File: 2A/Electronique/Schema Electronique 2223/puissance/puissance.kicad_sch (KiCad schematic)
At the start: 19 parts, among them J101 Bat 2, J102 Bat 1, J103 AU, J104 Switch, J15 Conn_02x20_Odd_Even

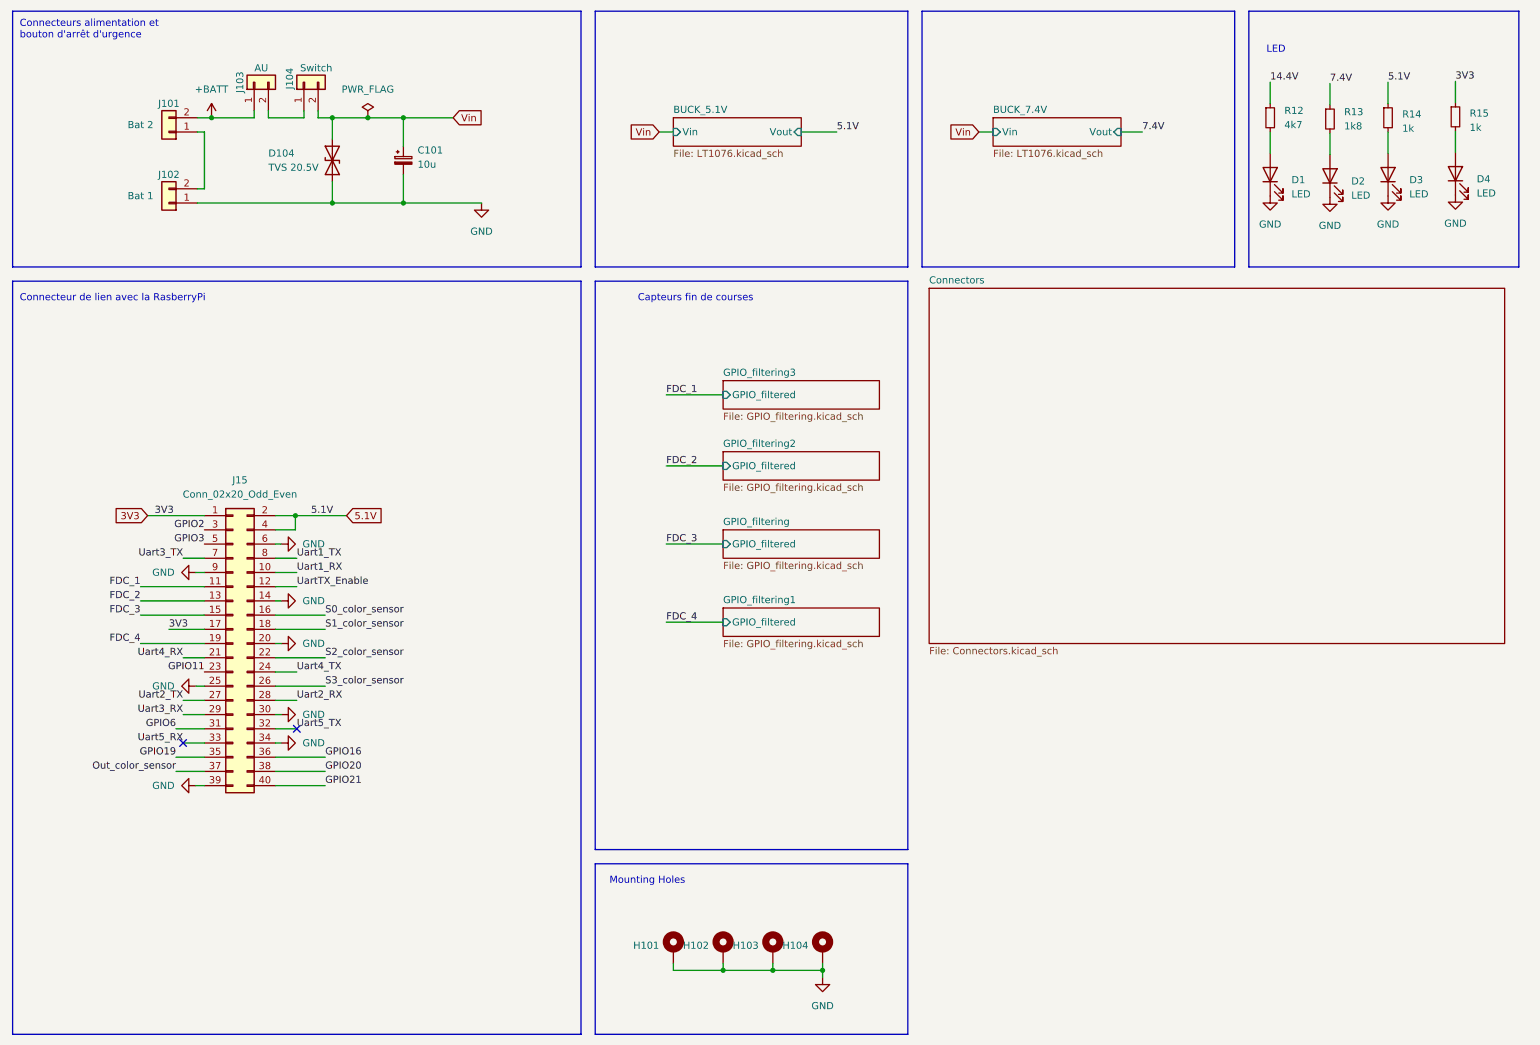
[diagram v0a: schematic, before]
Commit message: update puissance
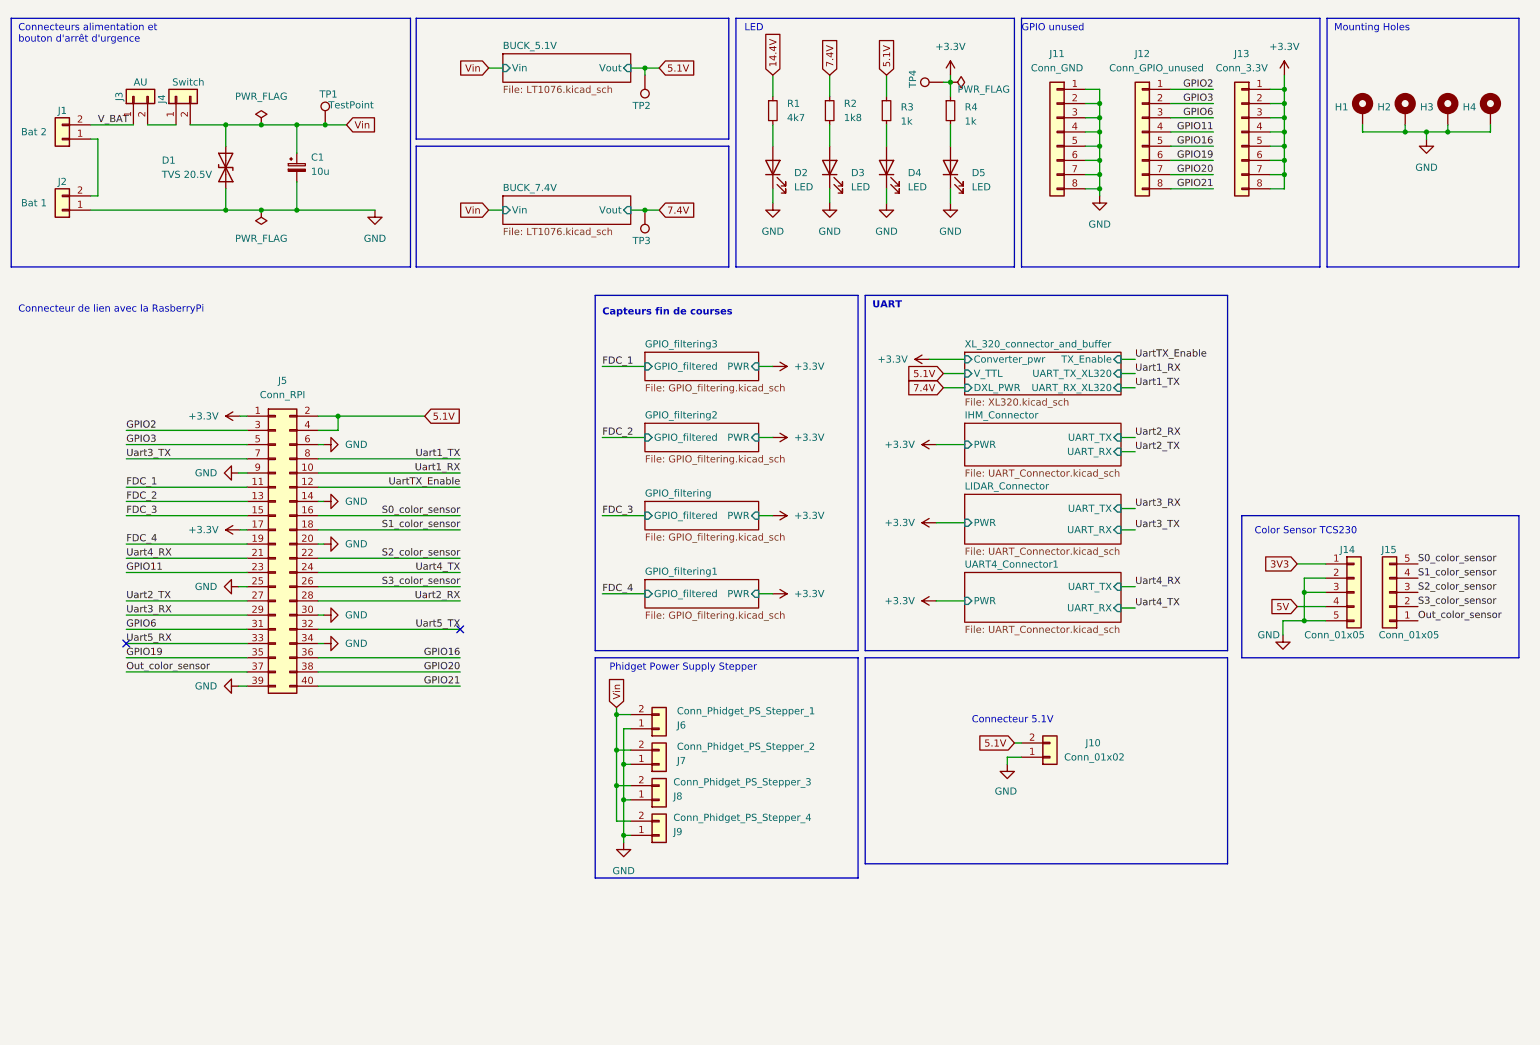
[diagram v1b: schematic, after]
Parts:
- removed C101: 10u, Capacitor_SMD:CP_Elec_5x5.4, symbol Device:C_Polarized_Small
- removed D1: LED, LED_SMD:LED_0603_1608Metric_Pad1.05x0.95mm_HandSolder, symbol Device:LED
- removed D104: TVS 20.5V, symbol Diode:1.5KExxCA
- removed H101, H102, H103, H104: MountingHole_Pad, MountingHole:MountingHole_3.2mm_M3_Pad_Via, symbol Mechanical:MountingHole_Pad
- removed J101: Bat 2, symbol Connector_Generic:Conn_01x02
- removed J102: Bat 1, symbol Connector_Generic:Conn_01x02
- removed J103: AU, symbol Connector_Generic:Conn_01x02
- removed J104: Switch, symbol Connector_Generic:Conn_01x02
- removed J15: Conn_02x20_Odd_Even, symbol Connector_Generic:Conn_02x20_Odd_Even
- removed R12: 4k7, Resistor_SMD:R_0603_1608Metric_Pad0.98x0.95mm_HandSolder, symbol Device:R_Small
- removed R13: 1k8, Resistor_SMD:R_0603_1608Metric_Pad0.98x0.95mm_HandSolder, symbol Device:R_Small
- removed R14, R15: 1k, Resistor_SMD:R_0603_1608Metric_Pad0.98x0.95mm_HandSolder, symbol Device:R_Small
- added C1: 10u, Capacitor_SMD:CP_Elec_4x5.4, symbol Device:C_Polarized_Small
- added D1: TVS 20.5V, Diode_SMD:D_SMB, symbol Diode:1.5KExxCA
- added D5: LED, LED_SMD:LED_0603_1608Metric, symbol Device:LED
- added H1, H2, H3, H4: MountingHole_Pad, MountingHole:MountingHole_2.7mm_M2.5_Pad_Via, symbol Mechanical:MountingHole_Pad
- added J1: Bat 2, custom:691322110002, symbol Connector_Generic:Conn_01x02
- added J10: Conn_01x02, Connector_JST:JST_XH_B2B-XH-A_1x02_P2.50mm_Vertical, symbol Connector_Generic:Conn_01x02
- added J11: Conn_GND, Connector_PinHeader_2.54mm:PinHeader_1x08_P2.54mm_Vertical, symbol Connector_Generic:Conn_01x08
- added J12: Conn_GPIO_unused, Connector_PinHeader_2.54mm:PinHeader_1x08_P2.54mm_Vertical, symbol Connector_Generic:Conn_01x08
- added J13: Conn_3.3V, Connector_PinHeader_2.54mm:PinHeader_1x08_P2.54mm_Vertical, symbol Connector_Generic:Conn_01x08
- added J14, J15: Conn_01x05, Connector_JST:JST_XH_B5B-XH-A_1x05_P2.50mm_Vertical, symbol Connector_Generic:Conn_01x05
- added J2: Bat 1, custom:691322110002, symbol Connector_Generic:Conn_01x02
- added J3: AU, custom:691322110002, symbol Connector_Generic:Conn_01x02
- added J4: Switch, custom:691322110002, symbol Connector_Generic:Conn_01x02
- added J5: Conn_RPI, Connector_PinSocket_2.54mm:PinSocket_2x20_P2.54mm_Vertical, symbol Connector_Generic:Conn_02x20_Odd_Even
- added J6: Conn_Phidget_PS_Stepper_1, Connector_JST:JST_XH_B2B-XH-A_1x02_P2.50mm_Vertical, symbol Connector_Generic:Conn_01x02
- added J7: Conn_Phidget_PS_Stepper_2, Connector_JST:JST_XH_B2B-XH-A_1x02_P2.50mm_Vertical, symbol Connector_Generic:Conn_01x02
- added J8: Conn_Phidget_PS_Stepper_3, Connector_JST:JST_XH_B2B-XH-A_1x02_P2.50mm_Vertical, symbol Connector_Generic:Conn_01x02
- added J9: Conn_Phidget_PS_Stepper_4, Connector_JST:JST_XH_B2B-XH-A_1x02_P2.50mm_Vertical, symbol Connector_Generic:Conn_01x02
- added R1: 4k7, Resistor_SMD:R_0402_1005Metric, symbol Device:R_Small
- added R2: 1k8, Resistor_SMD:R_0402_1005Metric, symbol Device:R_Small
- added R3, R4: 1k, Resistor_SMD:R_0402_1005Metric, symbol Device:R_Small
- added TP1: TestPoint, Connector_Pin:Pin_D0.9mm_L10.0mm_W2.4mm_FlatFork, symbol Connector:TestPoint
- added TP2: 5.1V, Connector_Pin:Pin_D0.9mm_L10.0mm_W2.4mm_FlatFork, symbol Connector:TestPoint
- added TP3: 7.4V, Connector_Pin:Pin_D0.9mm_L10.0mm_W2.4mm_FlatFork, symbol Connector:TestPoint
- added TP4: 3V3, Connector_Pin:Pin_D0.9mm_L10.0mm_W2.4mm_FlatFork, symbol Connector:TestPoint
- D2, D3, D4: footprint LED_SMD:LED_0603_1608Metric_Pad1.05x0.95mm_HandSolder -> LED_SMD:LED_0603_1608Metric
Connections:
- net 14.4V: now also R1.1
- net 3V3: now also J14.1 (Pin_1)
- net 5.1V: now also J10.2 (Pin_2), J5.2 (Pin_2), J5.4 (Pin_4), R3.1, TP2.1
- net 7.4V: now also R2.1, TP3.1
- net FDC_1: now also J5.11 (Pin_11)
- net FDC_2: now also J5.13 (Pin_13)
- net FDC_3: now also J5.15 (Pin_15)
- net FDC_4: now also J5.19 (Pin_19)
- net GND: now also C1.2, D1.2 (A2), D5.1 (K), H1.1, H2.1, H3.1, H4.1, J10.1 (Pin_1), J11.1 (Pin_1), J11.2 (Pin_2), J11.3 (Pin_3), J11.4 (Pin_4), J11.5 (Pin_5), J11.6 (Pin_6), J11.7 (Pin_7), J11.8 (Pin_8), J14.2 (Pin_2), J14.3 (Pin_3), J14.5 (Pin_5), J2.1 (Pin_1), J5.14 (Pin_14), J5.20 (Pin_20), J5.25 (Pin_25), J5.30 (Pin_30), J5.34 (Pin_34), J5.39 (Pin_39), J5.6 (Pin_6), J5.9 (Pin_9), J6.1 (Pin_1), J7.1 (Pin_1), J8.1 (Pin_1), J9.1 (Pin_1)
- net GPIO11: now also J12.4 (Pin_4), J5.23 (Pin_23)
- net GPIO16: now also J12.5 (Pin_5), J5.36 (Pin_36)
- net GPIO19: now also J12.6 (Pin_6), J5.35 (Pin_35)
- net GPIO2: now also J12.1 (Pin_1), J5.3 (Pin_3)
- net GPIO20: now also J12.7 (Pin_7), J5.38 (Pin_38)
- net GPIO21: now also J12.8 (Pin_8), J5.40 (Pin_40)
- net GPIO3: now also J12.2 (Pin_2), J5.5 (Pin_5)
- net GPIO6: now also J12.3 (Pin_3), J5.31 (Pin_31)
- net Out_color_sensor: now also J15.1 (Pin_1), J5.37 (Pin_37)
- net S0_color_sensor: now also J15.5 (Pin_5), J5.16 (Pin_16)
- net S1_color_sensor: now also J15.4 (Pin_4), J5.18 (Pin_18)
- net S2_color_sensor: now also J15.3 (Pin_3), J5.22 (Pin_22)
- net S3_color_sensor: now also J15.2 (Pin_2), J5.26 (Pin_26)
- net Uart1_RX: now also J5.10 (Pin_10)
- net Uart1_TX: now also J5.8 (Pin_8)
- net Uart2_RX: now also J5.28 (Pin_28)
- net Uart2_TX: now also J5.27 (Pin_27)
- net Uart3_RX: now also J5.29 (Pin_29)
- net Uart3_TX: now also J5.7 (Pin_7)
- net Uart4_RX: now also J5.21 (Pin_21)
- net Uart4_TX: now also J5.24 (Pin_24)
- net Uart5_RX: now also J5.33 (Pin_33)
- net Uart5_TX: now also J5.32 (Pin_32)
- net UartTX_Enable: now also J5.12 (Pin_12)
- net Vin: now also C1.1, D1.1 (A1), J4.2 (Pin_2), J6.2 (Pin_2), J7.2 (Pin_2), J8.2 (Pin_2), J9.2 (Pin_2), TP1.1
- net at D3.2 (A): now also R2.2
- net at D2.2 (A): now also R1.2
- net at D4.2 (A): now also R3.2
- new net: J3.2 (Pin_2), J4.1 (Pin_1)
- new net: D5.2 (A), R4.2
- new net: J1.1 (Pin_1), J2.2 (Pin_2)
- new net +3.3V: J13.1 (Pin_1), J13.2 (Pin_2), J13.3 (Pin_3), J13.4 (Pin_4), J13.5 (Pin_5), J13.6 (Pin_6), J13.7 (Pin_7), J13.8 (Pin_8), J5.1 (Pin_1), J5.17 (Pin_17), R4.1, TP4.1
- new net 5V: J14.4 (Pin_4)
- new net V_BAT: J1.2 (Pin_2), J3.1 (Pin_1)
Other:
- removed sheet Connectors
- added sheet IHM_Connector (UART_Connector.kicad_sch)
- added sheet LIDAR_Connector (UART_Connector.kicad_sch)
- added sheet UART4_Connector1 (UART_Connector.kicad_sch)
- added sheet XL_320_connector_and_buffer (XL320.kicad_sch)
- sheet GPIO_filtering ports: added PWR; removed none
- sheet GPIO_filtering1 ports: added PWR; removed none
- sheet GPIO_filtering2 ports: added PWR; removed none
- sheet GPIO_filtering3 ports: added PWR; removed none
- note added: "Color Sensor TCS230"
- note added: "Connecteur 5.1V"
- note added: "GPIO unused"
- note added: "Phidget Power Supply Stepper"
- note added: "UART"
